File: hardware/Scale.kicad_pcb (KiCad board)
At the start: 2 copper layers, 58.2 x 25.9 mm, 45 parts, among them J1 Load Cell Connector, J2 DebugEdge_02x03, J3 Display Connector, J4 GPIO, J5 RS232, J6 USB_C_Receptacle, Q1 DMG2307L, Q2 DMG2307L, Q3 BSD235N, SW1 RESET, SW2 PEC12R Encoder, U1 STM32G070CBTx_u, U3 MCP6N11-010, U4 MCP4542, U5 AP9101CK, U6 MIC5504-3.3YM5, X1 KC2520Z

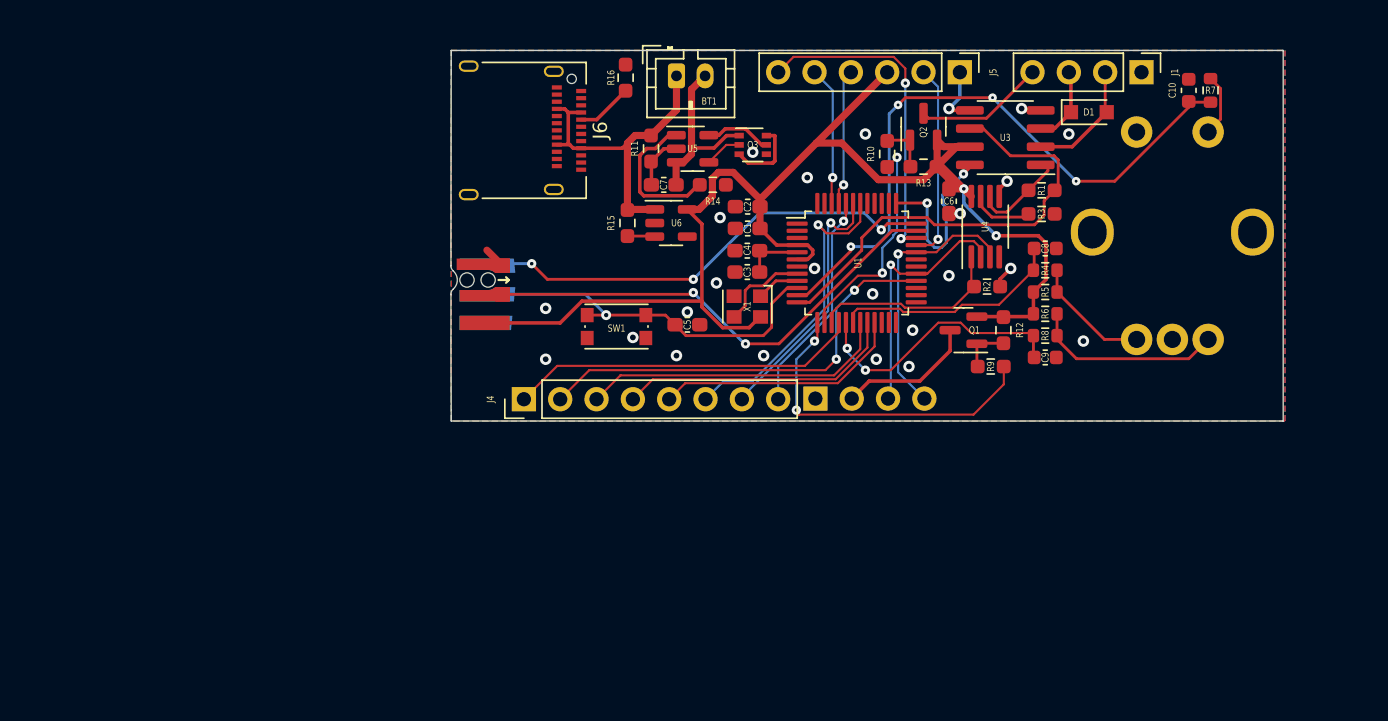
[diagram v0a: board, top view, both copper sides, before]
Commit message: Started on pcb
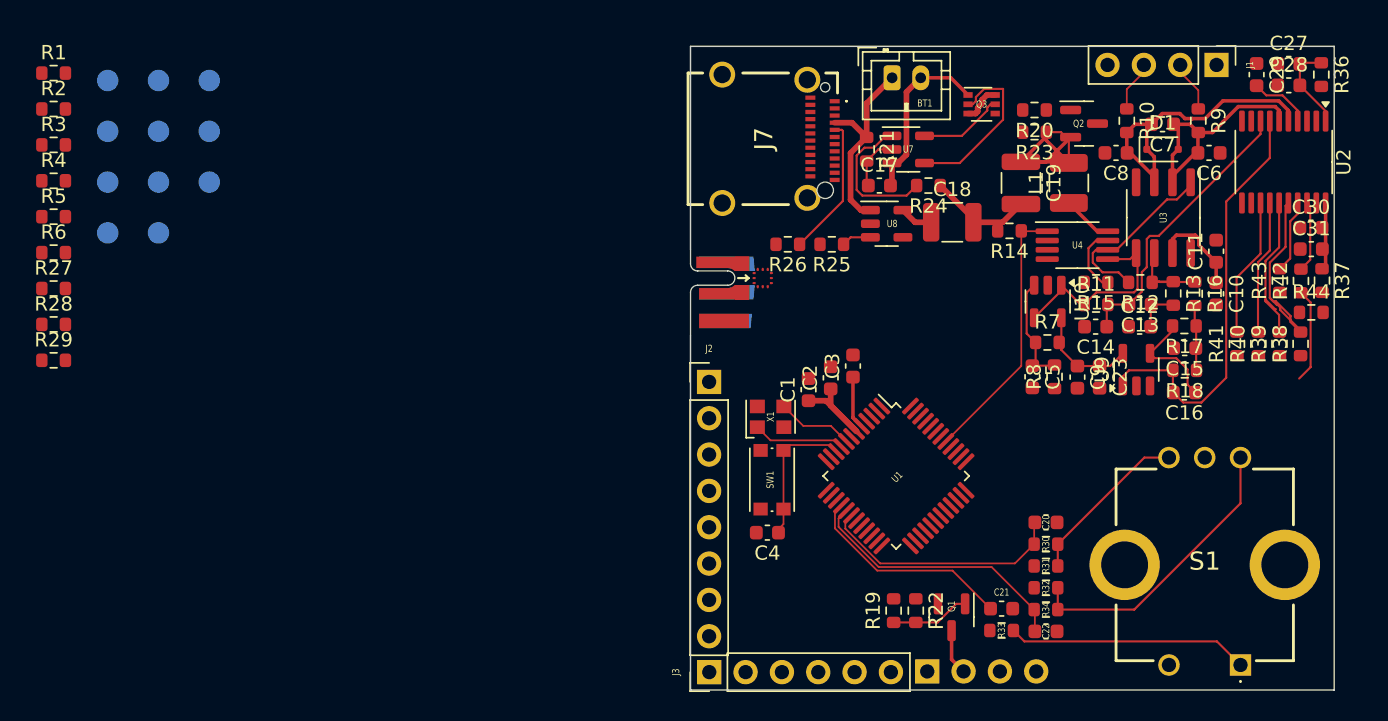
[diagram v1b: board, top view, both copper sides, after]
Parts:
- removed the C4 at (117.2, 60.7)
- removed J6: USB_C_Receptacle, Custom:USB_C_Receptacle_Amphenol_12401610E4-2A
- removed SW2: PEC12R Encoder, Custom:Bourns PEC12R Vertical
- added C10: 1uF, Capacitor_SMD:C_0603_1608Metric, F.Cu at (150.0, 63.8)
- added C12: 1uF, Capacitor_SMD:C_0603_1608Metric, F.Cu at (144.7, 66.0)
- added C13: 1uF, Capacitor_SMD:C_0603_1608Metric, F.Cu at (144.7, 64.5)
- added C14: 1uF, Capacitor_SMD:C_0603_1608Metric, F.Cu at (141.6, 66.0)
- added C15: 220nF, Capacitor_SMD:C_0603_1608Metric, F.Cu at (147.8, 67.5)
- added C16: 47nF, Capacitor_SMD:C_0603_1608Metric, F.Cu at (147.8, 70.6)
- added C18: 10uF, Capacitor_SMD:C_1210_3225Metric, F.Cu at (131.6, 58.8)
- added C19: 10uF, Capacitor_SMD:C_1210_3225Metric, F.Cu at (136.3, 56.0)
- added C23: 100nF, Capacitor_SMD:C_0603_1608Metric, F.Cu at (141.8, 69.6)
- added C27: 100nF, Capacitor_SMD:C_0603_1608Metric, F.Cu at (155.1, 47.7)
- added C28: 100nF, Capacitor_SMD:C_0603_1608Metric, F.Cu at (155.1, 49.2)
- added C29: 10uF, Capacitor_SMD:C_0603_1608Metric, F.Cu at (152.8, 48.4)
- added C30: 100nF, Capacitor_SMD:C_0603_1608Metric, F.Cu at (156.6, 59.1)
- added C31: 100nF, Capacitor_SMD:C_0603_1608Metric, F.Cu at (156.7, 60.6)
- added C5: 100nF, Capacitor_SMD:C_0603_1608Metric, F.Cu at (137.2, 69.5)
- added C6: 10nF, Capacitor_SMD:C_0603_1608Metric, F.Cu at (149.5, 53.9)
- added C7: 100nF, Capacitor_SMD:C_0603_1608Metric, F.Cu at (146.2, 51.9)
- added C8: 10nF, Capacitor_SMD:C_0603_1608Metric, F.Cu at (143.0, 53.9)
- added C9: 100nF, Capacitor_SMD:C_0603_1608Metric, F.Cu at (140.3, 69.6)
- added J7: 12401610E4#2A, custom:12401610E42A, F.Cu at (118.3, 52.9)
- added L1: 10uH, Inductor_SMD:L_1210_3225Metric, F.Cu at (139.7, 56.0)
- added R1: 1.0K 1%, Resistor_SMD:R_0603_1608Metric, F.Cu at (68.7, 48.3)
- added R10: 20k 1%, Resistor_SMD:R_0603_1608Metric, F.Cu at (143.8, 51.6)
- added R11: 20k 1%, Resistor_SMD:R_0603_1608Metric, F.Cu at (141.6, 64.5)
- added R13: 20k 1%, Resistor_SMD:R_0603_1608Metric, F.Cu at (147.0, 63.7)
- added R16: 20k 1%, Resistor_SMD:R_0603_1608Metric, F.Cu at (148.5, 63.8)
- added R17: 10k 1%, Resistor_SMD:R_0603_1608Metric, F.Cu at (147.8, 66.0)
- added R18: 20k 1%, Resistor_SMD:R_0603_1608Metric, F.Cu at (147.8, 69.1)
- added R2: 1.0K 1%, Resistor_SMD:R_0603_1608Metric, F.Cu at (68.7, 50.8)
- added R27: 1K, Resistor_SMD:R_0603_1608Metric, F.Cu at (68.7, 63.4)
- added R28: 1K, Resistor_SMD:R_0603_1608Metric, F.Cu at (68.7, 65.9)
- added R29: 1K, Resistor_SMD:R_0603_1608Metric, F.Cu at (68.7, 68.4)
- added R3: 1.0K 1%, Resistor_SMD:R_0603_1608Metric, F.Cu at (68.7, 53.3)
- added R36: 10R 1%, Resistor_SMD:R_0603_1608Metric, F.Cu at (157.3, 48.4)
- added R37: 10R 1%, Resistor_SMD:R_0603_1608Metric, F.Cu at (157.4, 62.8)
- added R38: 10R 1%, Resistor_SMD:R_0603_1608Metric, F.Cu at (155.9, 67.2)
- added R39: 10R 1%, Resistor_SMD:R_0603_1608Metric, F.Cu at (154.4, 67.2)
- added R4: 1.0K 1%, Resistor_SMD:R_0603_1608Metric, F.Cu at (68.7, 55.9)
- added R40: 10R 1%, Resistor_SMD:R_0603_1608Metric, F.Cu at (152.9, 67.2)
- added R41: 10R 1%, Resistor_SMD:R_0603_1608Metric, F.Cu at (151.4, 67.2)
- added R42: 10R 1%, Resistor_SMD:R_0603_1608Metric, F.Cu at (155.9, 62.9)
- added R43: 10R 1%, Resistor_SMD:R_0603_1608Metric, F.Cu at (154.4, 62.8)
- added R44: 10K 1%, Resistor_SMD:R_0603_1608Metric, F.Cu at (156.7, 65.0)
- added R5: 1.0K 1%, Resistor_SMD:R_0603_1608Metric, F.Cu at (68.7, 58.4)
- added R6: 1.0K 1%, Resistor_SMD:R_0603_1608Metric, F.Cu at (68.7, 60.9)
- added R7: 100k 1%, Resistor_SMD:R_0603_1608Metric, F.Cu at (138.2, 67.2)
- added R8: 100k 1%, Resistor_SMD:R_0603_1608Metric, F.Cu at (138.7, 69.5)
- added R9: 20k 1%, Resistor_SMD:R_0603_1608Metric, F.Cu at (148.8, 51.6)
- added S1: PEC12R-3217F-S0024, custom:PEC12R3217FS0024, F.Cu at (151.7, 89.7)
- added TP1: TP_INA_OUT_UNFILTERED, TestPoint:TestPoint_Pad_D1.5mm, B.Cu at (72.5, 48.8)
- added TP2: TP_ADC_VREF, TestPoint:TestPoint_Pad_D1.5mm, B.Cu at (72.5, 52.4)
- added TP3: TP_INA_OUT_ACTIVE, TestPoint:TestPoint_Pad_D1.5mm, B.Cu at (72.5, 55.9)
- added TP4: TP_INA_OUT_FILTERED_PASSIVE, TestPoint:TestPoint_Pad_D1.5mm, B.Cu at (72.5, 59.5)
- added TP5: TP_INA_IN_P, TestPoint:TestPoint_Pad_D1.5mm, B.Cu at (76.1, 48.8)
- added TP6: TP_INA_IN_N, TestPoint:TestPoint_Pad_D1.5mm, B.Cu at (76.1, 52.4)
- added TP_3V1: TP_3V3, TestPoint:TestPoint_Pad_D1.5mm, B.Cu at (76.1, 55.9)
- added TP_3V3A1: TP_3V3A, TestPoint:TestPoint_Pad_D1.5mm, B.Cu at (76.1, 59.5)
- added TP_BAT_N1: TP_BAT_N, TestPoint:TestPoint_Pad_D1.5mm, B.Cu at (79.6, 48.8)
- added TP_GND1: TP_GND, TestPoint:TestPoint_Pad_D1.5mm, B.Cu at (79.6, 52.4)
- added TP_VDD1: TP_VDD, TestPoint:TestPoint_Pad_D1.5mm, B.Cu at (79.6, 55.9)
- added U10: MCP6001-OT, Package_TO_SOT_SMD:SOT-23-5, F.Cu at (138.2, 64.3)
- added U2: MCP3562R-E/ST, Package_SO:TSSOP-20_4.4x6.5mm_P0.65mm, F.Cu at (154.7, 54.5)
- added U9: MCP6001-OT, Package_TO_SOT_SMD:SOT-23-5, F.Cu at (144.4, 69.0)
- C1, C2, C3: footprint Capacitor_SMD:C_0603_1608Metric_Pad1.08x0.95mm_HandSolder -> Capacitor_SMD:C_0603_1608Metric
- C11: renamed from C6; footprint Capacitor_SMD:C_0603_1608Metric_Pad1.08x0.95mm_HandSolder -> Capacitor_SMD:C_0603_1608Metric
- C17: renamed from C7; footprint Capacitor_SMD:C_0603_1608Metric_Pad1.08x0.95mm_HandSolder -> Capacitor_SMD:C_0603_1608Metric
- C4: renamed from C5; footprint Capacitor_SMD:C_0603_1608Metric_Pad1.08x0.95mm_HandSolder -> Capacitor_SMD:C_0603_1608Metric
- D1: footprint Diode_SMD:D_SOD-323_HandSoldering -> Diode_SMD:D_SOD-323F
- J4: renamed from J2; footprint custom:DebugEdge_2x03_Target -> Connector_DebugEdge:DebugEdge_2x03_Target
- J5: renamed from J3; footprint Custom:0.96'' Display -> Connector_PinHeader_2.54mm:PinHeader_1x04_P2.54mm_Vertical
- R12: renamed from R1; footprint Resistor_SMD:R_0603_1608Metric_Pad0.98x0.95mm_HandSolder -> Resistor_SMD:R_0603_1608Metric
- R14: renamed from R2; footprint Resistor_SMD:R_0603_1608Metric_Pad0.98x0.95mm_HandSolder -> Resistor_SMD:R_0603_1608Metric
- R15: renamed from R3; footprint Resistor_SMD:R_0603_1608Metric_Pad0.98x0.95mm_HandSolder -> Resistor_SMD:R_0603_1608Metric
- R19: renamed from R9; footprint Resistor_SMD:R_0603_1608Metric_Pad0.98x0.95mm_HandSolder -> Resistor_SMD:R_0603_1608Metric
- R20: renamed from R10; footprint Resistor_SMD:R_0603_1608Metric_Pad0.98x0.95mm_HandSolder -> Resistor_SMD:R_0603_1608Metric
- R21: renamed from R11; footprint Resistor_SMD:R_0603_1608Metric_Pad0.98x0.95mm_HandSolder -> Resistor_SMD:R_0603_1608Metric
- R22: renamed from R12; footprint Resistor_SMD:R_0603_1608Metric_Pad0.98x0.95mm_HandSolder -> Resistor_SMD:R_0603_1608Metric
- R23: renamed from R13; footprint Resistor_SMD:R_0603_1608Metric_Pad0.98x0.95mm_HandSolder -> Resistor_SMD:R_0603_1608Metric
- R24: renamed from R14; footprint Resistor_SMD:R_0603_1608Metric_Pad0.98x0.95mm_HandSolder -> Resistor_SMD:R_0603_1608Metric
- R25: renamed from R15; footprint Resistor_SMD:R_0603_1608Metric_Pad0.98x0.95mm_HandSolder -> Resistor_SMD:R_0603_1608Metric
- R26: renamed from R16; footprint Resistor_SMD:R_0603_1608Metric_Pad0.98x0.95mm_HandSolder -> Resistor_SMD:R_0603_1608Metric
- moved J3 45.5 mm to (114.6, 90.2), turned to 90 degrees
- moved R33 40.5 mm to (135.0, 87.3), turned to 180 degrees
- moved C21 38.5 mm to (135.0, 85.8), turned to 0 degrees
- moved R22 20.5 mm to (129.0, 85.9)
- moved Q1 20.1 mm to (131.5, 86.4), turned to -90 degrees
- moved J5 19.5 mm to (129.8, 90.2), turned to -90 degrees
- moved R32 19.2 mm to (138.1, 84.3)
- moved C20 19.2 mm to (138.1, 79.7)
- moved R30 19.2 mm to (138.1, 81.3)
- moved R31 19.2 mm to (138.1, 82.8)
- moved C22 19.2 mm to (138.1, 87.3)
- moved R34 19.2 mm to (138.1, 85.8)
- moved C11 19.0 mm to (150.0, 60.8), turned to 90 degrees
- moved R19 18.4 mm to (127.5, 85.9), turned to 90 degrees
- moved J4 16.8 mm to (113.2, 63.6)
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- renumbered C8 to C20, C10 to C21, C9 to C22, J4 to J2, J5 to J3, R4 to R30, R5 to R31, R6 to R32, R7 to R33, R8 to R34, U5 to U7, U6 to U8
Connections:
- net /I2C_SCL renamed /Display/SCL
- net /I2C_SDA renamed /Display/SDA
- net /Instrumentation Amplifier/INA_OUT renamed /Instrumentation Amplifier/INA_OUT_UNFILTERED
- C11 pad 1: +3V3 -> +3.3VA
- C3 pad 1: /MCU/MCU_VREF -> +3.3VA
- D1 pad 1: /Instrumentation Amplifier/BRIDGE_B -> /Instrumentation Amplifier/INA_IN_P
- D1 pad 2: /Instrumentation Amplifier/BRIDGE_A -> /Instrumentation Amplifier/INA_IN_N
- J2 pad 1: /MCU/GPIO_PA5 -> /MCU/GPIO_PB7
- Q2 pad 2: +3V3 -> +3.3VA
- R23 pad 1: +3V3 -> +3.3VA
- R25 pad 1: +BATT -> /MCU/LDO_EN
- R25 pad 2: Net-(R15-Pad2) -> GND
- U1 pad 1: unconnected-(U1-Pad1) -> /ADC/ADC_IRQ
- U1 pad 11: /Encoder/ENCODER_BUTTON -> /ADC/ADC_VREF
- U1 pad 13: /MCU/DISPLAY_ENABLE -> /Instrumentation Amplifier/INA_OUT_FILTERED_PASSIVE
- U1 pad 14: /MCU/BRIDGE_ENABLE -> /ADC/INA_OUT_FILTERED_ACTIVE
- U1 pad 15: /Instrumentation Amplifier/DPOT_HVC_A0 -> unconnected-(U1A-PA4/ADC1_IN4/I2S1_WS/RTC_OUT_ALARM/RTC_OUT_CALIB/SPI1_NSS/SPI2_MOSI/TIM14_CH1-Pad15)
- U1 pad 16: /MCU/GPIO_PA5 -> /Encoder/ENCODER_BUTTON
- U1 pad 22: unconnected-(U1-Pad22) -> /MCU/DISPLAY_ENABLE
- U1 pad 23: unconnected-(U1-Pad23) -> /MCU/BRIDGE_ENABLE
- U1 pad 24: unconnected-(U1-Pad24) -> /ADC/~{SS}
- U1 pad 25: unconnected-(U1-Pad25) -> /ADC/CLK
- U1 pad 26: unconnected-(U1-Pad26) -> /ADC/MISO
- U1 pad 27: unconnected-(U1-Pad27) -> /ADC/MOSI
- U1 pad 3: unconnected-(U1-Pad3) -> /MCU/LDO_EN
- U1 pad 4: +3V3 -> +BATT
- U1 pad 40: unconnected-(U1-Pad40) -> /ADC/ADC_MCLK
- U1 pad 41: unconnected-(U1-Pad41) -> /Instrumentation Amplifier/DPOT_HVC_A0
- U1 pad 45: /MCU/USART_TX -> /MCU/GPIO_PB5
- U1 pad 46: /MCU/USART_RX -> /MCU/GPIO_PB7
- U1 pad 47: unconnected-(U1-Pad47) -> /MCU/USART_TX
- U1 pad 48: unconnected-(U1-Pad48) -> /MCU/USART_RX
- U1 pad 5: /MCU/MCU_VREF -> +3.3VA
- U3 pad 2: /Instrumentation Amplifier/BRIDGE_A -> /Instrumentation Amplifier/INA_IN_N
- U3 pad 3: /Instrumentation Amplifier/BRIDGE_B -> /Instrumentation Amplifier/INA_IN_P
- U3 pad 5: GND -> /Instrumentation Amplifier/INA_VREF
- U3 pad 7: +3V3 -> +3.3VA
- U4 pad 5: GND -> /Instrumentation Amplifier/INA_VREF
- U8 pad 3: Net-(R15-Pad2) -> /MCU/LDO_EN
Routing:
- net +3V3: track 102.3 -> 13.8 mm, vias 2 -> 0
- net /MCU/SWDIO: track 33.7 -> 0.00 mm, vias 2 -> 0
- net +3.3VA: track 0.00 -> 33.7 mm
- net /MCU/SWDCLK: track 33.3 -> 0.00 mm, vias 3 -> 0
- net /MCU/GPIO_PA8: track 30.4 -> 0.00 mm, vias 2 -> 0
- net /Encoder/ENCODER_BUTTON: track 44.6 -> 14.4 mm, vias 4 -> 0
- net /ADC/INA_OUT_FILTERED_ACTIVE: track 0.00 -> 29.8 mm
- net /Instrumentation Amplifier/INA_OUT_UNFILTERED: track 31.7 -> 5.83 mm
- net /MCU/GPIO_PA5: track 24.0 -> 0.00 mm
- net /MCU/DISPLAY_ENABLE: track 23.7 -> 0.00 mm, vias 2 -> 0
- net /MCU/USART_RTS: track 22.7 -> 0.00 mm, vias 2 -> 0
- net /MCU/GPIO_PB3: track 21.8 -> 0.00 mm, vias 1 -> 0
- net /MCU/GPIO_PB0: track 21.8 -> 0.00 mm
- net /Instrumentation Amplifier/INA_IN_P: track 0.00 -> 21.7 mm
- net /ADC/ADC_VREF: track 0.00 -> 19.9 mm
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- removed copper zone on B.Cu, net GND
- removed copper zone on F.Cu, net GND
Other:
- board size 58.2 x 25.9 mm -> 45 x 45 mm
